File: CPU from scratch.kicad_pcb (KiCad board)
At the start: 2 copper layers, 90 x 35 mm, 50 parts, among them J1 Screw_Terminal_01x03, J2 Screw_Terminal_01x02, Q1 2N3904, Q10 2N3904, Q11 2N3904, Q12 2N3904, Q13 2N3904, Q14 2N3904, Q15 2N3904, Q16 2N3904, Q17 2N3904, Q18 2N3904, Q19 2N3904, Q2 2N3904, Q20 2N3904, Q21 2N3904, Q3 2N3904, Q4 2N3904, Q5 2N3904, Q6 2N3904, Q7 2N3904, Q8 2N3904, Q9 2N3904

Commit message: Update Readme
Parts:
- removed J1: Screw_Terminal_01x03, TerminalBlock_Phoenix:TerminalBlock_Phoenix_MKDS-1,5-3-5.08_1x03_P5.08mm_Horizontal
- removed J2: Screw_Terminal_01x02, TerminalBlock_Phoenix:TerminalBlock_Phoenix_MKDS-1,5-2-5.08_1x02_P5.08mm_Horizontal
- added D1: D, Diode_THT:D_DO-35_SOD27_P7.62mm_Horizontal, F.Cu at (136.9, 49.1)
- added D1: D, Diode_THT:D_DO-35_SOD27_P7.62mm_Horizontal, F.Cu at (136.9, 117.5)
- added D1: D, Diode_THT:D_DO-35_SOD27_P7.62mm_Horizontal, F.Cu at (149.3, 157.2)
- added D2: D, Diode_THT:D_DO-35_SOD27_P7.62mm_Horizontal, F.Cu at (124.9, 45.1)
- added D2: D, Diode_THT:D_DO-35_SOD27_P7.62mm_Horizontal, F.Cu at (161.3, 161.2)
- added D2: D, Diode_THT:D_DO-35_SOD27_P7.62mm_Horizontal, F.Cu at (124.9, 113.5)
- added D3: D, Diode_THT:D_DO-35_SOD27_P7.62mm_Horizontal, F.Cu at (160.6, 141.4)
- added D3: D, Diode_THT:D_DO-35_SOD27_P7.62mm_Horizontal, F.Cu at (125.6, 64.9)
- added D3: D, Diode_THT:D_DO-35_SOD27_P7.62mm_Horizontal, F.Cu at (125.6, 133.3)
- added D4: D, Diode_THT:D_DO-35_SOD27_P7.62mm_Horizontal, F.Cu at (168.8, 48.9)
- added D4: D, Diode_THT:D_DO-35_SOD27_P7.62mm_Horizontal, F.Cu at (168.8, 117.3)
- added D4: D, Diode_THT:D_DO-35_SOD27_P7.62mm_Horizontal, F.Cu at (117.4, 157.4)
- added D5: D, Diode_THT:D_DO-35_SOD27_P7.62mm_Horizontal, F.Cu at (129.4, 161.4)
- added D5: D, Diode_THT:D_DO-35_SOD27_P7.62mm_Horizontal, F.Cu at (156.8, 113.3)
- added D5: D, Diode_THT:D_DO-35_SOD27_P7.62mm_Horizontal, F.Cu at (156.8, 44.9)
- added D6: D, Diode_THT:D_DO-35_SOD27_P7.62mm_Horizontal, F.Cu at (120.6, 141.4)
- added D6: D, Diode_THT:D_DO-35_SOD27_P7.62mm_Horizontal, F.Cu at (165.6, 133.3)
- added D6: D, Diode_THT:D_DO-35_SOD27_P7.62mm_Horizontal, F.Cu at (165.6, 64.9)
- added D7: D, Diode_THT:D_DO-35_SOD27_P7.62mm_Horizontal, F.Cu at (137.6, 141.4)
- added D7: D, Diode_THT:D_DO-35_SOD27_P7.62mm_Horizontal, F.Cu at (148.6, 64.9)
- added D7: D, Diode_THT:D_DO-35_SOD27_P7.62mm_Horizontal, F.Cu at (148.6, 133.3)
- added Q1: 2N3904, Package_TO_SOT_THT:TO-92_Inline, F.Cu at (144.3, 155.7)
- added Q1: 2N3904, Package_TO_SOT_THT:TO-92_Inline, F.Cu at (141.9, 119.0)
- added Q1: 2N3904, Package_TO_SOT_THT:TO-92_Inline, F.Cu at (141.9, 50.6)
- added Q10: 2N3904, Package_TO_SOT_THT:TO-92_Inline, F.Cu at (173.8, 50.3)
- added Q10: 2N3904, Package_TO_SOT_THT:TO-92_Inline, F.Cu at (112.4, 156.0)
- added Q10: 2N3904, Package_TO_SOT_THT:TO-92_Inline, F.Cu at (173.8, 118.7)
- added Q11: 2N3904, Package_TO_SOT_THT:TO-92_Inline, F.Cu at (121.4, 163.0)
- added Q11: 2N3904, Package_TO_SOT_THT:TO-92_Inline, F.Cu at (164.8, 111.7)
- added Q11: 2N3904, Package_TO_SOT_THT:TO-92_Inline, F.Cu at (164.8, 43.3)
- added Q12: 2N3904, Package_TO_SOT_THT:TO-92_Inline, F.Cu at (164.8, 117.7)
- added Q12: 2N3904, Package_TO_SOT_THT:TO-92_Inline, F.Cu at (121.4, 157.0)
- added Q12: 2N3904, Package_TO_SOT_THT:TO-92_Inline, F.Cu at (164.8, 49.3)
- added Q13: 2N3904, Package_TO_SOT_THT:TO-92_Inline, F.Cu at (157.5, 117.5)
- added Q13: 2N3904, Package_TO_SOT_THT:TO-92_Inline, F.Cu at (157.5, 49.1)
- added Q13: 2N3904, Package_TO_SOT_THT:TO-92_Inline, F.Cu at (128.7, 157.2)
- added Q14: 2N3904, Package_TO_SOT_THT:TO-92_Inline, F.Cu at (133.4, 163.0)
- added Q14: 2N3904, Package_TO_SOT_THT:TO-92_Inline, F.Cu at (152.8, 43.3)
- added Q14: 2N3904, Package_TO_SOT_THT:TO-92_Inline, F.Cu at (152.8, 111.7)
- added Q15: 2N3904, Package_TO_SOT_THT:TO-92_Inline, F.Cu at (152.8, 49.3)
- added Q15: 2N3904, Package_TO_SOT_THT:TO-92_Inline, F.Cu at (133.4, 157.0)
- added Q15: 2N3904, Package_TO_SOT_THT:TO-92_Inline, F.Cu at (152.8, 117.7)
- added Q16: 2N3904, Package_TO_SOT_THT:TO-92_Inline, F.Cu at (170.6, 134.8)
- added Q16: 2N3904, Package_TO_SOT_THT:TO-92_Inline, F.Cu at (115.6, 139.9)
- added Q16: 2N3904, Package_TO_SOT_THT:TO-92_Inline, F.Cu at (170.6, 66.4)
- added Q17: 2N3904, Package_TO_SOT_THT:TO-92_Inline, F.Cu at (161.6, 60.1)
- added Q17: 2N3904, Package_TO_SOT_THT:TO-92_Inline, F.Cu at (161.6, 128.5)
- added Q17: 2N3904, Package_TO_SOT_THT:TO-92_Inline, F.Cu at (124.6, 146.2)
- added Q18: 2N3904, Package_TO_SOT_THT:TO-92_Inline, F.Cu at (161.6, 66.4)
- added Q18: 2N3904, Package_TO_SOT_THT:TO-92_Inline, F.Cu at (161.6, 134.8)
- added Q18: 2N3904, Package_TO_SOT_THT:TO-92_Inline, F.Cu at (124.6, 139.9)
- added Q19: 2N3904, Package_TO_SOT_THT:TO-92_Inline, F.Cu at (153.5, 134.8)
- added Q19: 2N3904, Package_TO_SOT_THT:TO-92_Inline, F.Cu at (132.7, 139.9)
- added Q19: 2N3904, Package_TO_SOT_THT:TO-92_Inline, F.Cu at (153.5, 66.4)
- added Q2: 2N3904, Package_TO_SOT_THT:TO-92_Inline, F.Cu at (153.3, 162.7)
- added Q2: 2N3904, Package_TO_SOT_THT:TO-92_Inline, F.Cu at (132.9, 43.6)
- added Q2: 2N3904, Package_TO_SOT_THT:TO-92_Inline, F.Cu at (132.9, 112.0)
- added Q20: 2N3904, Package_TO_SOT_THT:TO-92_Inline, F.Cu at (144.6, 128.3)
- added Q20: 2N3904, Package_TO_SOT_THT:TO-92_Inline, F.Cu at (141.6, 146.4)
- added Q20: 2N3904, Package_TO_SOT_THT:TO-92_Inline, F.Cu at (144.6, 59.9)
- added Q21: 2N3904, Package_TO_SOT_THT:TO-92_Inline, F.Cu at (144.6, 65.9)
- added Q21: 2N3904, Package_TO_SOT_THT:TO-92_Inline, F.Cu at (141.6, 140.4)
- added Q21: 2N3904, Package_TO_SOT_THT:TO-92_Inline, F.Cu at (144.6, 134.3)
- added Q3: 2N3904, Package_TO_SOT_THT:TO-92_Inline, F.Cu at (132.9, 49.6)
- added Q3: 2N3904, Package_TO_SOT_THT:TO-92_Inline, F.Cu at (153.3, 156.7)
- added Q3: 2N3904, Package_TO_SOT_THT:TO-92_Inline, F.Cu at (132.9, 118.0)
- added Q4: 2N3904, Package_TO_SOT_THT:TO-92_Inline, F.Cu at (125.6, 49.3)
- added Q4: 2N3904, Package_TO_SOT_THT:TO-92_Inline, F.Cu at (125.6, 117.7)
- added Q4: 2N3904, Package_TO_SOT_THT:TO-92_Inline, F.Cu at (160.6, 157.0)
- added Q5: 2N3904, Package_TO_SOT_THT:TO-92_Inline, F.Cu at (165.3, 162.5)
- added Q5: 2N3904, Package_TO_SOT_THT:TO-92_Inline, F.Cu at (120.9, 43.8)
- added Q5: 2N3904, Package_TO_SOT_THT:TO-92_Inline, F.Cu at (120.9, 112.2)
- added Q6: 2N3904, Package_TO_SOT_THT:TO-92_Inline, F.Cu at (165.3, 156.5)
- added Q6: 2N3904, Package_TO_SOT_THT:TO-92_Inline, F.Cu at (120.9, 118.2)
- added Q6: 2N3904, Package_TO_SOT_THT:TO-92_Inline, F.Cu at (120.9, 49.8)
- added Q7: 2N3904, Package_TO_SOT_THT:TO-92_Inline, F.Cu at (155.6, 139.9)
- added Q7: 2N3904, Package_TO_SOT_THT:TO-92_Inline, F.Cu at (130.6, 66.4)
- added Q7: 2N3904, Package_TO_SOT_THT:TO-92_Inline, F.Cu at (130.6, 134.8)
- added Q8: 2N3904, Package_TO_SOT_THT:TO-92_Inline, F.Cu at (121.6, 60.1)
- added Q8: 2N3904, Package_TO_SOT_THT:TO-92_Inline, F.Cu at (121.6, 128.5)
- added Q8: 2N3904, Package_TO_SOT_THT:TO-92_Inline, F.Cu at (164.6, 146.2)
- added Q9: 2N3904, Package_TO_SOT_THT:TO-92_Inline, F.Cu at (121.6, 66.1)
- added Q9: 2N3904, Package_TO_SOT_THT:TO-92_Inline, F.Cu at (121.6, 134.5)
- added Q9: 2N3904, Package_TO_SOT_THT:TO-92_Inline, F.Cu at (164.6, 140.2)
- added R1: 1k, Resistor_THT:R_Axial_DIN0207_L6.3mm_D2.5mm_P7.62mm_Horizontal, F.Cu at (115.6, 40.3)
- added R1: 1k, Resistor_THT:R_Axial_DIN0207_L6.3mm_D2.5mm_P7.62mm_Horizontal, F.Cu at (170.6, 166.0)
- added R1: 1k, Resistor_THT:R_Axial_DIN0207_L6.3mm_D2.5mm_P7.62mm_Horizontal, F.Cu at (115.6, 108.7)
- added R10: 1k, Resistor_THT:R_Axial_DIN0207_L6.3mm_D2.5mm_P7.62mm_Horizontal, F.Cu at (114.1, 105.7)
- added R10: 1k, Resistor_THT:R_Axial_DIN0207_L6.3mm_D2.5mm_P7.62mm_Horizontal, F.Cu at (172.1, 169.0)
- added R10: 1k, Resistor_THT:R_Axial_DIN0207_L6.3mm_D2.5mm_P7.62mm_Horizontal, F.Cu at (114.1, 37.3)
- added R11: 1k, Resistor_THT:R_Axial_DIN0207_L6.3mm_D2.5mm_P7.62mm_Horizontal, F.Cu at (126.4, 54.1)
- added R11: 1k, Resistor_THT:R_Axial_DIN0207_L6.3mm_D2.5mm_P7.62mm_Horizontal, F.Cu at (159.7, 152.2)
- added R11: 1k, Resistor_THT:R_Axial_DIN0207_L6.3mm_D2.5mm_P7.62mm_Horizontal, F.Cu at (126.4, 122.5)
- added R12: 1k, Resistor_THT:R_Axial_DIN0207_L6.3mm_D2.5mm_P7.62mm_Horizontal, F.Cu at (130.6, 121.7)
- added R12: 1k, Resistor_THT:R_Axial_DIN0207_L6.3mm_D2.5mm_P7.62mm_Horizontal, F.Cu at (155.6, 153.0)
- added R12: 1k, Resistor_THT:R_Axial_DIN0207_L6.3mm_D2.5mm_P7.62mm_Horizontal, F.Cu at (130.6, 53.3)
- added R13: 1k, Resistor_THT:R_Axial_DIN0207_L6.3mm_D2.5mm_P7.62mm_Horizontal, F.Cu at (170.6, 37.1)
- added R13: 1k, Resistor_THT:R_Axial_DIN0207_L6.3mm_D2.5mm_P7.62mm_Horizontal, F.Cu at (115.6, 169.2)
- added R13: 1k, Resistor_THT:R_Axial_DIN0207_L6.3mm_D2.5mm_P7.62mm_Horizontal, F.Cu at (170.6, 105.5)
- added R14: 1k, Resistor_THT:R_Axial_DIN0207_L6.3mm_D2.5mm_P7.62mm_Horizontal, F.Cu at (173.8, 105.7)
- added R14: 1k, Resistor_THT:R_Axial_DIN0207_L6.3mm_D2.5mm_P7.62mm_Horizontal, F.Cu at (112.4, 169.1)
- added R14: 1k, Resistor_THT:R_Axial_DIN0207_L6.3mm_D2.5mm_P7.62mm_Horizontal, F.Cu at (173.8, 37.3)
- added R15: 1k, Resistor_THT:R_Axial_DIN0207_L6.3mm_D2.5mm_P7.62mm_Horizontal, F.Cu at (159.8, 105.7)
- added R15: 1k, Resistor_THT:R_Axial_DIN0207_L6.3mm_D2.5mm_P7.62mm_Horizontal, F.Cu at (126.4, 169.1)
- added R15: 1k, Resistor_THT:R_Axial_DIN0207_L6.3mm_D2.5mm_P7.62mm_Horizontal, F.Cu at (159.8, 37.3)
- added R16: 1k, Resistor_THT:R_Axial_DIN0207_L6.3mm_D2.5mm_P7.62mm_Horizontal, F.Cu at (140.2, 169.2)
- added R16: 1k, Resistor_THT:R_Axial_DIN0207_L6.3mm_D2.5mm_P7.62mm_Horizontal, F.Cu at (145.9, 105.5)
- added R16: 1k, Resistor_THT:R_Axial_DIN0207_L6.3mm_D2.5mm_P7.62mm_Horizontal, F.Cu at (145.9, 37.1)
- added R17: 1k, Resistor_THT:R_Axial_DIN0207_L6.3mm_D2.5mm_P7.62mm_Horizontal, F.Cu at (166.4, 54.2)
- added R17: 1k, Resistor_THT:R_Axial_DIN0207_L6.3mm_D2.5mm_P7.62mm_Horizontal, F.Cu at (166.4, 122.6)
- added R17: 1k, Resistor_THT:R_Axial_DIN0207_L6.3mm_D2.5mm_P7.62mm_Horizontal, F.Cu at (119.7, 152.1)
- added R18: 1k, Resistor_THT:R_Axial_DIN0207_L6.3mm_D2.5mm_P7.62mm_Horizontal, F.Cu at (170.6, 53.3)
- added R18: 1k, Resistor_THT:R_Axial_DIN0207_L6.3mm_D2.5mm_P7.62mm_Horizontal, F.Cu at (170.6, 121.7)
- added R18: 1k, Resistor_THT:R_Axial_DIN0207_L6.3mm_D2.5mm_P7.62mm_Horizontal, F.Cu at (115.6, 153.0)
- added R19: 1k, Resistor_THT:R_Axial_DIN0207_L6.3mm_D2.5mm_P7.62mm_Horizontal, F.Cu at (148.9, 54.1)
- added R19: 1k, Resistor_THT:R_Axial_DIN0207_L6.3mm_D2.5mm_P7.62mm_Horizontal, F.Cu at (137.2, 152.2)
- added R19: 1k, Resistor_THT:R_Axial_DIN0207_L6.3mm_D2.5mm_P7.62mm_Horizontal, F.Cu at (148.9, 122.5)
- added R2: 1k, Resistor_THT:R_Axial_DIN0207_L6.3mm_D2.5mm_P7.62mm_Horizontal, F.Cu at (111.6, 47.9)
- added R2: 1k, Resistor_THT:R_Axial_DIN0207_L6.3mm_D2.5mm_P7.62mm_Horizontal, F.Cu at (174.6, 158.4)
- added R2: 1k, Resistor_THT:R_Axial_DIN0207_L6.3mm_D2.5mm_P7.62mm_Horizontal, F.Cu at (111.6, 116.3)
- added R20: 1k, Resistor_THT:R_Axial_DIN0207_L6.3mm_D2.5mm_P7.62mm_Horizontal, F.Cu at (153.6, 121.7)
- added R20: 1k, Resistor_THT:R_Axial_DIN0207_L6.3mm_D2.5mm_P7.62mm_Horizontal, F.Cu at (132.6, 153.0)
- added R20: 1k, Resistor_THT:R_Axial_DIN0207_L6.3mm_D2.5mm_P7.62mm_Horizontal, F.Cu at (153.6, 53.3)
- added R3: 1k, Resistor_THT:R_Axial_DIN0207_L6.3mm_D2.5mm_P7.62mm_Horizontal, F.Cu at (147.1, 118.3)
- added R3: 1k, Resistor_THT:R_Axial_DIN0207_L6.3mm_D2.5mm_P7.62mm_Horizontal, F.Cu at (147.1, 49.9)
- added R3: 1k, Resistor_THT:R_Axial_DIN0207_L6.3mm_D2.5mm_P7.62mm_Horizontal, F.Cu at (139.1, 156.4)
- added R4: 1k, Resistor_THT:R_Axial_DIN0207_L6.3mm_D2.5mm_P7.62mm_Horizontal, F.Cu at (170.6, 154.0)
- added R4: 1k, Resistor_THT:R_Axial_DIN0207_L6.3mm_D2.5mm_P7.62mm_Horizontal, F.Cu at (115.6, 52.3)
- added R4: 1k, Resistor_THT:R_Axial_DIN0207_L6.3mm_D2.5mm_P7.62mm_Horizontal, F.Cu at (115.6, 120.7)
- added R5: 1k, Resistor_THT:R_Axial_DIN0207_L6.3mm_D2.5mm_P7.62mm_Horizontal, F.Cu at (174.6, 154.0)
- added R5: 1k, Resistor_THT:R_Axial_DIN0207_L6.3mm_D2.5mm_P7.62mm_Horizontal, F.Cu at (111.6, 120.7)
- added R5: 1k, Resistor_THT:R_Axial_DIN0207_L6.3mm_D2.5mm_P7.62mm_Horizontal, F.Cu at (111.6, 52.3)
- added R6: 1k, Resistor_THT:R_Axial_DIN0207_L6.3mm_D2.5mm_P7.62mm_Horizontal, F.Cu at (148.6, 148.5)
- added R6: 1k, Resistor_THT:R_Axial_DIN0207_L6.3mm_D2.5mm_P7.62mm_Horizontal, F.Cu at (137.6, 126.2)
- added R6: 1k, Resistor_THT:R_Axial_DIN0207_L6.3mm_D2.5mm_P7.62mm_Horizontal, F.Cu at (137.6, 57.8)
- added R7: 1k, Resistor_THT:R_Axial_DIN0207_L6.3mm_D2.5mm_P7.62mm_Horizontal, F.Cu at (138.7, 105.7)
- added R7: 1k, Resistor_THT:R_Axial_DIN0207_L6.3mm_D2.5mm_P7.62mm_Horizontal, F.Cu at (138.7, 37.3)
- added R7: 1k, Resistor_THT:R_Axial_DIN0207_L6.3mm_D2.5mm_P7.62mm_Horizontal, F.Cu at (147.5, 169.0)
- added R8: 1k, Resistor_THT:R_Axial_DIN0207_L6.3mm_D2.5mm_P7.62mm_Horizontal, F.Cu at (141.9, 37.5)
- added R8: 1k, Resistor_THT:R_Axial_DIN0207_L6.3mm_D2.5mm_P7.62mm_Horizontal, F.Cu at (141.9, 105.9)
- added R8: 1k, Resistor_THT:R_Axial_DIN0207_L6.3mm_D2.5mm_P7.62mm_Horizontal, F.Cu at (144.3, 168.8)
- added R9: 1k, Resistor_THT:R_Axial_DIN0207_L6.3mm_D2.5mm_P7.62mm_Horizontal, F.Cu at (158.3, 168.8)
- added R9: 1k, Resistor_THT:R_Axial_DIN0207_L6.3mm_D2.5mm_P7.62mm_Horizontal, F.Cu at (127.9, 105.9)
- added R9: 1k, Resistor_THT:R_Axial_DIN0207_L6.3mm_D2.5mm_P7.62mm_Horizontal, F.Cu at (127.9, 37.5)
- moved R5 70.2 mm to (174.6, 84.4), turned to 90 degrees
- moved R2 69.1 mm to (174.6, 88.7), turned to -90 degrees
- moved R10 66.0 mm to (172.1, 99.4), turned to 180 degrees
- moved Q16 64.6 mm to (115.6, 70.3), turned to -90 degrees
- moved Q9 64.1 mm to (164.6, 70.5), turned to -90 degrees
- moved R4 62.4 mm to (170.6, 84.4), turned to 90 degrees
- moved R1 61.7 mm to (170.6, 96.4), turned to 90 degrees
- moved R14 57.7 mm to (112.4, 99.4), turned to 90 degrees
- moved Q8 57.1 mm to (164.6, 76.5), turned to -90 degrees
- moved D3 56.5 mm to (160.6, 71.7), turned to -90 degrees
- moved Q10 56.3 mm to (112.4, 86.3), turned to -90 degrees
- moved D6 55.3 mm to (120.6, 71.7), turned to -90 degrees
- moved Q18 52.3 mm to (124.6, 70.3), turned to -90 degrees
- moved Q7 52.1 mm to (155.6, 70.3), turned to -90 degrees
- moved R13 51.8 mm to (115.6, 99.6), turned to 0 degrees
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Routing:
- net /AND2/In1: track 42.7 -> 170.9 mm, vias 1 -> 4
- net /AND1/O: track 35.7 -> 142.7 mm
- net Cin: track 50.1 -> 133.4 mm
- net /XOR1/In2: track 24.8 -> 99.4 mm
- net GND: track 0.00 -> 68.1 mm
- net Net-(Q11-E): track 22.4 -> 89.8 mm
- net /XOR2/In2: track 20.7 -> 82.9 mm
- net /XOR1/In1: track 20.6 -> 82.6 mm
- net Net-(D6-A): track 15.9 -> 63.5 mm
- net Net-(D1-A): track 15.8 -> 63.4 mm
- net Net-(D4-A): track 15.7 -> 62.7 mm
- net Net-(Q2-E): track 14.8 -> 59.1 mm
- net /AND1/In2: track 12.0 -> 48.2 mm
- net /AND2/O: track 11.6 -> 46.6 mm
- net Net-(D3-A): track 8.74 -> 34.9 mm
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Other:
- board size 90 x 35 mm -> 76.2 x 144.8 mm
- board text added: "${REFERENCE}"

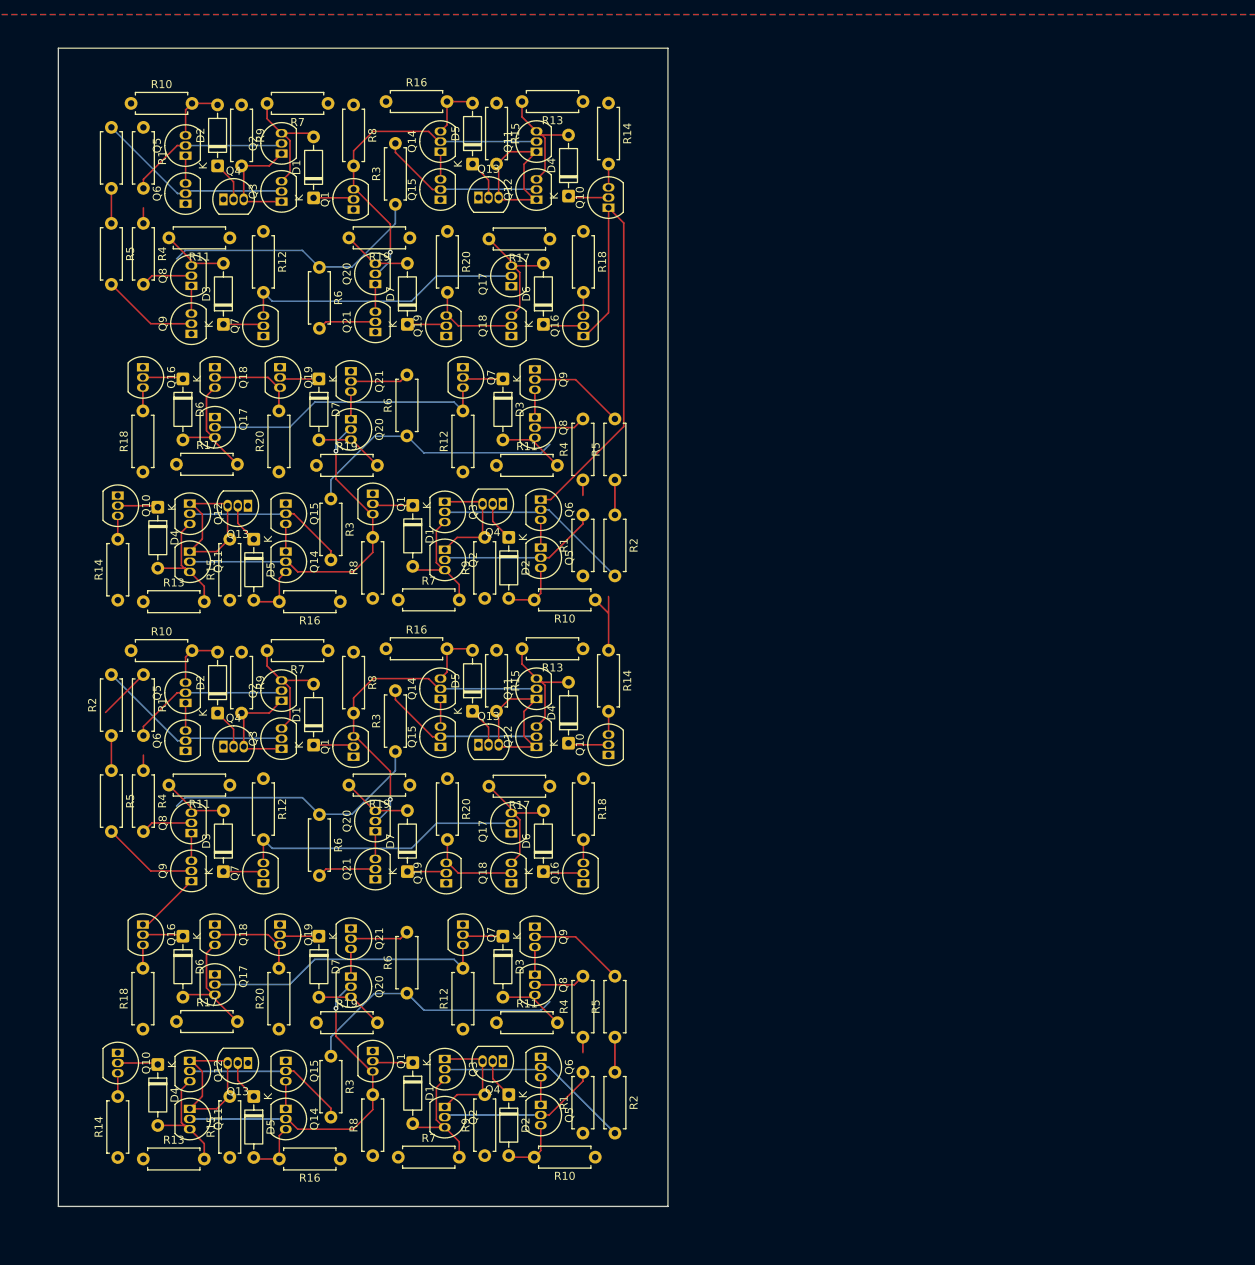
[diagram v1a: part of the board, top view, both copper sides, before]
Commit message: Update Readme
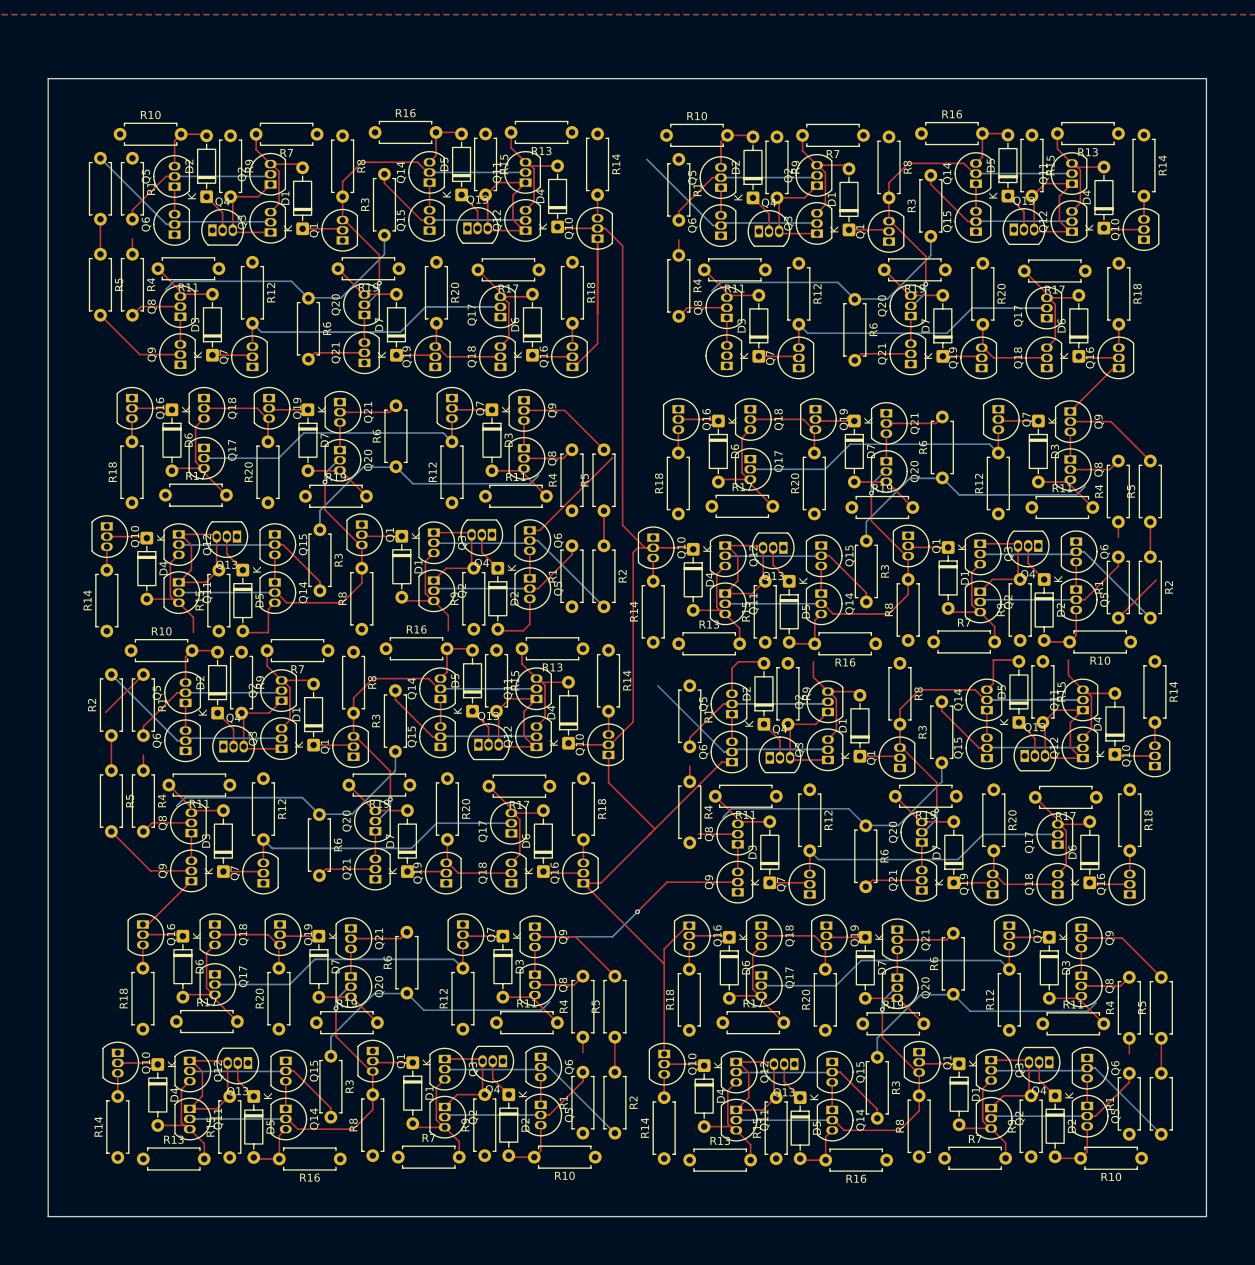
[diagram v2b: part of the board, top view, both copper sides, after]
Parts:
- removed the R10 at (172.1, 99.4)
- removed the R13 at (115.6, 99.6)
- removed the R16 at (140.2, 99.6)
- removed the R7 at (147.5, 99.4)
- added D1: D, Diode_THT:D_DO-35_SOD27_P7.62mm_Horizontal, F.Cu at (217.6, 157.3)
- added D1: D, Diode_THT:D_DO-35_SOD27_P7.62mm_Horizontal, F.Cu at (203.8, 53.1)
- added D1: D, Diode_THT:D_DO-35_SOD27_P7.62mm_Horizontal, F.Cu at (216.2, 92.8)
- added D1: D, Diode_THT:D_DO-35_SOD27_P7.62mm_Horizontal, F.Cu at (205.2, 118.9)
- added D2: D, Diode_THT:D_DO-35_SOD27_P7.62mm_Horizontal, F.Cu at (228.2, 96.8)
- added D2: D, Diode_THT:D_DO-35_SOD27_P7.62mm_Horizontal, F.Cu at (191.8, 49.1)
- added D2: D, Diode_THT:D_DO-35_SOD27_P7.62mm_Horizontal, F.Cu at (193.2, 114.9)
- added D2: D, Diode_THT:D_DO-35_SOD27_P7.62mm_Horizontal, F.Cu at (229.6, 161.3)
- added D3: D, Diode_THT:D_DO-35_SOD27_P7.62mm_Horizontal, F.Cu at (192.5, 68.9)
- added D3: D, Diode_THT:D_DO-35_SOD27_P7.62mm_Horizontal, F.Cu at (193.9, 134.7)
- added D3: D, Diode_THT:D_DO-35_SOD27_P7.62mm_Horizontal, F.Cu at (228.9, 141.5)
- added D3: D, Diode_THT:D_DO-35_SOD27_P7.62mm_Horizontal, F.Cu at (227.5, 77.0)
- added D4: D, Diode_THT:D_DO-35_SOD27_P7.62mm_Horizontal, F.Cu at (237.1, 118.7)
- added D4: D, Diode_THT:D_DO-35_SOD27_P7.62mm_Horizontal, F.Cu at (185.7, 157.6)
- added D4: D, Diode_THT:D_DO-35_SOD27_P7.62mm_Horizontal, F.Cu at (235.7, 52.9)
- added D4: D, Diode_THT:D_DO-35_SOD27_P7.62mm_Horizontal, F.Cu at (184.3, 93.0)
- added D5: D, Diode_THT:D_DO-35_SOD27_P7.62mm_Horizontal, F.Cu at (223.7, 48.9)
- added D5: D, Diode_THT:D_DO-35_SOD27_P7.62mm_Horizontal, F.Cu at (196.3, 97.0)
- added D5: D, Diode_THT:D_DO-35_SOD27_P7.62mm_Horizontal, F.Cu at (225.1, 114.7)
- added D5: D, Diode_THT:D_DO-35_SOD27_P7.62mm_Horizontal, F.Cu at (197.7, 161.6)
- added D6: D, Diode_THT:D_DO-35_SOD27_P7.62mm_Horizontal, F.Cu at (188.9, 141.5)
- added D6: D, Diode_THT:D_DO-35_SOD27_P7.62mm_Horizontal, F.Cu at (233.9, 134.7)
- added D6: D, Diode_THT:D_DO-35_SOD27_P7.62mm_Horizontal, F.Cu at (187.5, 77.0)
- added D6: D, Diode_THT:D_DO-35_SOD27_P7.62mm_Horizontal, F.Cu at (232.5, 68.9)
- added D7: D, Diode_THT:D_DO-35_SOD27_P7.62mm_Horizontal, F.Cu at (204.5, 77.0)
- added D7: D, Diode_THT:D_DO-35_SOD27_P7.62mm_Horizontal, F.Cu at (216.9, 134.7)
- added D7: D, Diode_THT:D_DO-35_SOD27_P7.62mm_Horizontal, F.Cu at (215.5, 68.9)
- added D7: D, Diode_THT:D_DO-35_SOD27_P7.62mm_Horizontal, F.Cu at (205.9, 141.5)
- added Q1: 2N3904, Package_TO_SOT_THT:TO-92_Inline, F.Cu at (208.8, 54.6)
- added Q1: 2N3904, Package_TO_SOT_THT:TO-92_Inline, F.Cu at (211.2, 91.3)
- added Q1: 2N3904, Package_TO_SOT_THT:TO-92_Inline, F.Cu at (210.2, 120.4)
- added Q1: 2N3904, Package_TO_SOT_THT:TO-92_Inline, F.Cu at (212.6, 155.9)
- added Q10: 2N3904, Package_TO_SOT_THT:TO-92_Inline, F.Cu at (242.1, 120.1)
- added Q10: 2N3904, Package_TO_SOT_THT:TO-92_Inline, F.Cu at (179.3, 91.6)
- added Q10: 2N3904, Package_TO_SOT_THT:TO-92_Inline, F.Cu at (180.7, 156.1)
- added Q10: 2N3904, Package_TO_SOT_THT:TO-92_Inline, F.Cu at (240.7, 54.3)
- added Q11: 2N3904, Package_TO_SOT_THT:TO-92_Inline, F.Cu at (189.7, 163.1)
- added Q11: 2N3904, Package_TO_SOT_THT:TO-92_Inline, F.Cu at (188.3, 98.6)
- added Q11: 2N3904, Package_TO_SOT_THT:TO-92_Inline, F.Cu at (231.7, 47.3)
- added Q11: 2N3904, Package_TO_SOT_THT:TO-92_Inline, F.Cu at (233.1, 113.1)
- added Q12: 2N3904, Package_TO_SOT_THT:TO-92_Inline, F.Cu at (188.3, 92.6)
- added Q12: 2N3904, Package_TO_SOT_THT:TO-92_Inline, F.Cu at (231.7, 53.3)
- added Q12: 2N3904, Package_TO_SOT_THT:TO-92_Inline, F.Cu at (233.1, 119.1)
- added Q12: 2N3904, Package_TO_SOT_THT:TO-92_Inline, F.Cu at (189.7, 157.1)
- added Q13: 2N3904, Package_TO_SOT_THT:TO-92_Inline, F.Cu at (225.8, 118.9)
- added Q13: 2N3904, Package_TO_SOT_THT:TO-92_Inline, F.Cu at (224.4, 53.1)
- added Q13: 2N3904, Package_TO_SOT_THT:TO-92_Inline, F.Cu at (197.0, 157.4)
- added Q13: 2N3904, Package_TO_SOT_THT:TO-92_Inline, F.Cu at (195.6, 92.8)
- added Q14: 2N3904, Package_TO_SOT_THT:TO-92_Inline, F.Cu at (221.1, 113.1)
- added Q14: 2N3904, Package_TO_SOT_THT:TO-92_Inline, F.Cu at (200.3, 98.6)
- added Q14: 2N3904, Package_TO_SOT_THT:TO-92_Inline, F.Cu at (201.7, 163.1)
- added Q14: 2N3904, Package_TO_SOT_THT:TO-92_Inline, F.Cu at (219.7, 47.3)
- added Q15: 2N3904, Package_TO_SOT_THT:TO-92_Inline, F.Cu at (219.7, 53.3)
- added Q15: 2N3904, Package_TO_SOT_THT:TO-92_Inline, F.Cu at (221.1, 119.1)
- added Q15: 2N3904, Package_TO_SOT_THT:TO-92_Inline, F.Cu at (201.7, 157.1)
- added Q15: 2N3904, Package_TO_SOT_THT:TO-92_Inline, F.Cu at (200.3, 92.6)
- added Q16: 2N3904, Package_TO_SOT_THT:TO-92_Inline, F.Cu at (183.9, 140.1)
- added Q16: 2N3904, Package_TO_SOT_THT:TO-92_Inline, F.Cu at (237.5, 70.4)
- added Q16: 2N3904, Package_TO_SOT_THT:TO-92_Inline, F.Cu at (238.9, 136.2)
- added Q16: 2N3904, Package_TO_SOT_THT:TO-92_Inline, F.Cu at (182.5, 75.5)
- added Q17: 2N3904, Package_TO_SOT_THT:TO-92_Inline, F.Cu at (229.9, 129.9)
- added Q17: 2N3904, Package_TO_SOT_THT:TO-92_Inline, F.Cu at (191.5, 81.8)
- added Q17: 2N3904, Package_TO_SOT_THT:TO-92_Inline, F.Cu at (192.9, 146.3)
- added Q17: 2N3904, Package_TO_SOT_THT:TO-92_Inline, F.Cu at (228.5, 64.1)
- added Q18: 2N3904, Package_TO_SOT_THT:TO-92_Inline, F.Cu at (229.9, 136.2)
- added Q18: 2N3904, Package_TO_SOT_THT:TO-92_Inline, F.Cu at (191.5, 75.5)
- added Q18: 2N3904, Package_TO_SOT_THT:TO-92_Inline, F.Cu at (192.9, 140.1)
- added Q18: 2N3904, Package_TO_SOT_THT:TO-92_Inline, F.Cu at (228.5, 70.4)
- added Q19: 2N3904, Package_TO_SOT_THT:TO-92_Inline, F.Cu at (220.4, 70.4)
- added Q19: 2N3904, Package_TO_SOT_THT:TO-92_Inline, F.Cu at (221.8, 136.2)
- added Q19: 2N3904, Package_TO_SOT_THT:TO-92_Inline, F.Cu at (201.0, 140.1)
- added Q19: 2N3904, Package_TO_SOT_THT:TO-92_Inline, F.Cu at (199.6, 75.5)
- added Q2: 2N3904, Package_TO_SOT_THT:TO-92_Inline, F.Cu at (220.2, 98.3)
- added Q2: 2N3904, Package_TO_SOT_THT:TO-92_Inline, F.Cu at (199.8, 47.6)
- added Q2: 2N3904, Package_TO_SOT_THT:TO-92_Inline, F.Cu at (201.2, 113.4)
- added Q2: 2N3904, Package_TO_SOT_THT:TO-92_Inline, F.Cu at (221.6, 162.9)
- added Q20: 2N3904, Package_TO_SOT_THT:TO-92_Inline, F.Cu at (211.5, 63.9)
- added Q20: 2N3904, Package_TO_SOT_THT:TO-92_Inline, F.Cu at (208.5, 82.0)
- added Q20: 2N3904, Package_TO_SOT_THT:TO-92_Inline, F.Cu at (212.9, 129.7)
- added Q20: 2N3904, Package_TO_SOT_THT:TO-92_Inline, F.Cu at (209.9, 146.6)
- added Q21: 2N3904, Package_TO_SOT_THT:TO-92_Inline, F.Cu at (209.9, 140.6)
- added Q21: 2N3904, Package_TO_SOT_THT:TO-92_Inline, F.Cu at (212.9, 135.7)
- added Q21: 2N3904, Package_TO_SOT_THT:TO-92_Inline, F.Cu at (211.5, 69.9)
- added Q21: 2N3904, Package_TO_SOT_THT:TO-92_Inline, F.Cu at (208.5, 76.0)
- added Q3: 2N3904, Package_TO_SOT_THT:TO-92_Inline, F.Cu at (201.2, 119.4)
- added Q3: 2N3904, Package_TO_SOT_THT:TO-92_Inline, F.Cu at (221.6, 156.9)
- added Q3: 2N3904, Package_TO_SOT_THT:TO-92_Inline, F.Cu at (199.8, 53.6)
- added Q3: 2N3904, Package_TO_SOT_THT:TO-92_Inline, F.Cu at (220.2, 92.3)
- added Q4: 2N3904, Package_TO_SOT_THT:TO-92_Inline, F.Cu at (228.9, 157.2)
- added Q4: 2N3904, Package_TO_SOT_THT:TO-92_Inline, F.Cu at (193.9, 119.1)
- added Q4: 2N3904, Package_TO_SOT_THT:TO-92_Inline, F.Cu at (227.5, 92.6)
- added Q4: 2N3904, Package_TO_SOT_THT:TO-92_Inline, F.Cu at (192.5, 53.3)
- added Q5: 2N3904, Package_TO_SOT_THT:TO-92_Inline, F.Cu at (187.8, 47.8)
- added Q5: 2N3904, Package_TO_SOT_THT:TO-92_Inline, F.Cu at (189.2, 113.6)
- added Q5: 2N3904, Package_TO_SOT_THT:TO-92_Inline, F.Cu at (233.6, 162.6)
- added Q5: 2N3904, Package_TO_SOT_THT:TO-92_Inline, F.Cu at (232.2, 98.1)
- added Q6: 2N3904, Package_TO_SOT_THT:TO-92_Inline, F.Cu at (233.6, 156.6)
- added Q6: 2N3904, Package_TO_SOT_THT:TO-92_Inline, F.Cu at (187.8, 53.8)
- added Q6: 2N3904, Package_TO_SOT_THT:TO-92_Inline, F.Cu at (232.2, 92.1)
- added Q6: 2N3904, Package_TO_SOT_THT:TO-92_Inline, F.Cu at (189.2, 119.6)
- added Q7: 2N3904, Package_TO_SOT_THT:TO-92_Inline, F.Cu at (198.9, 136.2)
- added Q7: 2N3904, Package_TO_SOT_THT:TO-92_Inline, F.Cu at (222.5, 75.5)
- added Q7: 2N3904, Package_TO_SOT_THT:TO-92_Inline, F.Cu at (197.5, 70.4)
- added Q7: 2N3904, Package_TO_SOT_THT:TO-92_Inline, F.Cu at (223.9, 140.1)
- added Q8: 2N3904, Package_TO_SOT_THT:TO-92_Inline, F.Cu at (232.9, 146.3)
- added Q8: 2N3904, Package_TO_SOT_THT:TO-92_Inline, F.Cu at (189.9, 129.9)
- added Q8: 2N3904, Package_TO_SOT_THT:TO-92_Inline, F.Cu at (188.5, 64.1)
- added Q8: 2N3904, Package_TO_SOT_THT:TO-92_Inline, F.Cu at (231.5, 81.8)
- added Q9: 2N3904, Package_TO_SOT_THT:TO-92_Inline, F.Cu at (232.9, 140.3)
- added Q9: 2N3904, Package_TO_SOT_THT:TO-92_Inline, F.Cu at (189.9, 135.9)
- added Q9: 2N3904, Package_TO_SOT_THT:TO-92_Inline, F.Cu at (231.5, 75.8)
- added Q9: 2N3904, Package_TO_SOT_THT:TO-92_Inline, F.Cu at (188.5, 70.1)
- added R1: 1k, Resistor_THT:R_Axial_DIN0207_L6.3mm_D2.5mm_P7.62mm_Horizontal, F.Cu at (182.5, 44.3)
- added R1: 1k, Resistor_THT:R_Axial_DIN0207_L6.3mm_D2.5mm_P7.62mm_Horizontal, F.Cu at (183.9, 110.1)
- added R1: 1k, Resistor_THT:R_Axial_DIN0207_L6.3mm_D2.5mm_P7.62mm_Horizontal, F.Cu at (237.5, 101.6)
- added R1: 1k, Resistor_THT:R_Axial_DIN0207_L6.3mm_D2.5mm_P7.62mm_Horizontal, F.Cu at (238.9, 166.2)
- added R10: 1k, Resistor_THT:R_Axial_DIN0207_L6.3mm_D2.5mm_P7.62mm_Horizontal, F.Cu at (239.0, 104.6)
- added R10: 1k, Resistor_THT:R_Axial_DIN0207_L6.3mm_D2.5mm_P7.62mm_Horizontal, F.Cu at (181.0, 41.3)
- added R10: 1k, Resistor_THT:R_Axial_DIN0207_L6.3mm_D2.5mm_P7.62mm_Horizontal, F.Cu at (240.4, 169.2)
- added R11: 1k, Resistor_THT:R_Axial_DIN0207_L6.3mm_D2.5mm_P7.62mm_Horizontal, F.Cu at (228.0, 152.3)
- added R11: 1k, Resistor_THT:R_Axial_DIN0207_L6.3mm_D2.5mm_P7.62mm_Horizontal, F.Cu at (193.4, 58.1)
- added R11: 1k, Resistor_THT:R_Axial_DIN0207_L6.3mm_D2.5mm_P7.62mm_Horizontal, F.Cu at (226.7, 87.8)
- added R11: 1k, Resistor_THT:R_Axial_DIN0207_L6.3mm_D2.5mm_P7.62mm_Horizontal, F.Cu at (194.7, 123.9)
- added R12: 1k, Resistor_THT:R_Axial_DIN0207_L6.3mm_D2.5mm_P7.62mm_Horizontal, F.Cu at (197.5, 57.3)
- added R12: 1k, Resistor_THT:R_Axial_DIN0207_L6.3mm_D2.5mm_P7.62mm_Horizontal, F.Cu at (222.5, 88.6)
- added R12: 1k, Resistor_THT:R_Axial_DIN0207_L6.3mm_D2.5mm_P7.62mm_Horizontal, F.Cu at (223.9, 153.2)
- added R12: 1k, Resistor_THT:R_Axial_DIN0207_L6.3mm_D2.5mm_P7.62mm_Horizontal, F.Cu at (198.9, 123.1)
- added R13: 1k, Resistor_THT:R_Axial_DIN0207_L6.3mm_D2.5mm_P7.62mm_Horizontal, F.Cu at (183.9, 169.4)
- added R13: 1k, Resistor_THT:R_Axial_DIN0207_L6.3mm_D2.5mm_P7.62mm_Horizontal, F.Cu at (237.5, 41.1)
- added R13: 1k, Resistor_THT:R_Axial_DIN0207_L6.3mm_D2.5mm_P7.62mm_Horizontal, F.Cu at (182.5, 104.8)
- added R14: 1k, Resistor_THT:R_Axial_DIN0207_L6.3mm_D2.5mm_P7.62mm_Horizontal, F.Cu at (240.7, 41.3)
- added R14: 1k, Resistor_THT:R_Axial_DIN0207_L6.3mm_D2.5mm_P7.62mm_Horizontal, F.Cu at (242.1, 107.1)
- added R14: 1k, Resistor_THT:R_Axial_DIN0207_L6.3mm_D2.5mm_P7.62mm_Horizontal, F.Cu at (179.3, 104.7)
- added R14: 1k, Resistor_THT:R_Axial_DIN0207_L6.3mm_D2.5mm_P7.62mm_Horizontal, F.Cu at (180.7, 169.2)
- added R15: 1k, Resistor_THT:R_Axial_DIN0207_L6.3mm_D2.5mm_P7.62mm_Horizontal, F.Cu at (226.7, 41.3)
- added R15: 1k, Resistor_THT:R_Axial_DIN0207_L6.3mm_D2.5mm_P7.62mm_Horizontal, F.Cu at (228.1, 107.1)
- added R15: 1k, Resistor_THT:R_Axial_DIN0207_L6.3mm_D2.5mm_P7.62mm_Horizontal, F.Cu at (194.7, 169.2)
- added R15: 1k, Resistor_THT:R_Axial_DIN0207_L6.3mm_D2.5mm_P7.62mm_Horizontal, F.Cu at (193.3, 104.7)
- added R16: 1k, Resistor_THT:R_Axial_DIN0207_L6.3mm_D2.5mm_P7.62mm_Horizontal, F.Cu at (208.5, 169.4)
- added R16: 1k, Resistor_THT:R_Axial_DIN0207_L6.3mm_D2.5mm_P7.62mm_Horizontal, F.Cu at (207.2, 104.8)
- added R16: 1k, Resistor_THT:R_Axial_DIN0207_L6.3mm_D2.5mm_P7.62mm_Horizontal, F.Cu at (212.9, 41.1)
- added R17: 1k, Resistor_THT:R_Axial_DIN0207_L6.3mm_D2.5mm_P7.62mm_Horizontal, F.Cu at (233.4, 58.2)
- added R17: 1k, Resistor_THT:R_Axial_DIN0207_L6.3mm_D2.5mm_P7.62mm_Horizontal, F.Cu at (188.0, 152.2)
- added R17: 1k, Resistor_THT:R_Axial_DIN0207_L6.3mm_D2.5mm_P7.62mm_Horizontal, F.Cu at (234.7, 124.0)
- added R17: 1k, Resistor_THT:R_Axial_DIN0207_L6.3mm_D2.5mm_P7.62mm_Horizontal, F.Cu at (186.7, 87.7)
- added R18: 1k, Resistor_THT:R_Axial_DIN0207_L6.3mm_D2.5mm_P7.62mm_Horizontal, F.Cu at (237.5, 57.3)
- added R18: 1k, Resistor_THT:R_Axial_DIN0207_L6.3mm_D2.5mm_P7.62mm_Horizontal, F.Cu at (182.5, 88.6)
- added R18: 1k, Resistor_THT:R_Axial_DIN0207_L6.3mm_D2.5mm_P7.62mm_Horizontal, F.Cu at (238.9, 123.1)
- added R18: 1k, Resistor_THT:R_Axial_DIN0207_L6.3mm_D2.5mm_P7.62mm_Horizontal, F.Cu at (183.9, 153.2)
- added R19: 1k, Resistor_THT:R_Axial_DIN0207_L6.3mm_D2.5mm_P7.62mm_Horizontal, F.Cu at (204.2, 87.8)
- added R19: 1k, Resistor_THT:R_Axial_DIN0207_L6.3mm_D2.5mm_P7.62mm_Horizontal, F.Cu at (215.9, 58.1)
- added R19: 1k, Resistor_THT:R_Axial_DIN0207_L6.3mm_D2.5mm_P7.62mm_Horizontal, F.Cu at (217.2, 123.9)
- added R19: 1k, Resistor_THT:R_Axial_DIN0207_L6.3mm_D2.5mm_P7.62mm_Horizontal, F.Cu at (205.5, 152.3)
- added R2: 1k, Resistor_THT:R_Axial_DIN0207_L6.3mm_D2.5mm_P7.62mm_Horizontal, F.Cu at (241.5, 94.0)
- added R2: 1k, Resistor_THT:R_Axial_DIN0207_L6.3mm_D2.5mm_P7.62mm_Horizontal, F.Cu at (242.9, 158.5)
- added R20: 1k, Resistor_THT:R_Axial_DIN0207_L6.3mm_D2.5mm_P7.62mm_Horizontal, F.Cu at (199.5, 88.6)
- added R20: 1k, Resistor_THT:R_Axial_DIN0207_L6.3mm_D2.5mm_P7.62mm_Horizontal, F.Cu at (221.9, 123.1)
- added R20: 1k, Resistor_THT:R_Axial_DIN0207_L6.3mm_D2.5mm_P7.62mm_Horizontal, F.Cu at (200.9, 153.2)
- added R20: 1k, Resistor_THT:R_Axial_DIN0207_L6.3mm_D2.5mm_P7.62mm_Horizontal, F.Cu at (220.5, 57.3)
- added R3: 1k, Resistor_THT:R_Axial_DIN0207_L6.3mm_D2.5mm_P7.62mm_Horizontal, F.Cu at (207.4, 156.5)
- added R3: 1k, Resistor_THT:R_Axial_DIN0207_L6.3mm_D2.5mm_P7.62mm_Horizontal, F.Cu at (206.0, 92.0)
- added R3: 1k, Resistor_THT:R_Axial_DIN0207_L6.3mm_D2.5mm_P7.62mm_Horizontal, F.Cu at (215.4, 119.7)
- added R3: 1k, Resistor_THT:R_Axial_DIN0207_L6.3mm_D2.5mm_P7.62mm_Horizontal, F.Cu at (214.0, 53.9)
- added R4: 1k, Resistor_THT:R_Axial_DIN0207_L6.3mm_D2.5mm_P7.62mm_Horizontal, F.Cu at (237.5, 89.6)
- added R4: 1k, Resistor_THT:R_Axial_DIN0207_L6.3mm_D2.5mm_P7.62mm_Horizontal, F.Cu at (183.9, 122.1)
- added R4: 1k, Resistor_THT:R_Axial_DIN0207_L6.3mm_D2.5mm_P7.62mm_Horizontal, F.Cu at (238.9, 154.2)
- added R4: 1k, Resistor_THT:R_Axial_DIN0207_L6.3mm_D2.5mm_P7.62mm_Horizontal, F.Cu at (182.5, 56.3)
- added R5: 1k, Resistor_THT:R_Axial_DIN0207_L6.3mm_D2.5mm_P7.62mm_Horizontal, F.Cu at (242.9, 154.2)
- added R5: 1k, Resistor_THT:R_Axial_DIN0207_L6.3mm_D2.5mm_P7.62mm_Horizontal, F.Cu at (241.5, 89.6)
- added R6: 1k, Resistor_THT:R_Axial_DIN0207_L6.3mm_D2.5mm_P7.62mm_Horizontal, F.Cu at (215.5, 84.1)
- added R6: 1k, Resistor_THT:R_Axial_DIN0207_L6.3mm_D2.5mm_P7.62mm_Horizontal, F.Cu at (205.9, 127.6)
- added R6: 1k, Resistor_THT:R_Axial_DIN0207_L6.3mm_D2.5mm_P7.62mm_Horizontal, F.Cu at (204.5, 61.8)
- added R6: 1k, Resistor_THT:R_Axial_DIN0207_L6.3mm_D2.5mm_P7.62mm_Horizontal, F.Cu at (216.9, 148.7)
- added R7: 1k, Resistor_THT:R_Axial_DIN0207_L6.3mm_D2.5mm_P7.62mm_Horizontal, F.Cu at (215.8, 169.2)
- added R7: 1k, Resistor_THT:R_Axial_DIN0207_L6.3mm_D2.5mm_P7.62mm_Horizontal, F.Cu at (214.4, 104.6)
- added R7: 1k, Resistor_THT:R_Axial_DIN0207_L6.3mm_D2.5mm_P7.62mm_Horizontal, F.Cu at (205.6, 41.3)
- added R8: 1k, Resistor_THT:R_Axial_DIN0207_L6.3mm_D2.5mm_P7.62mm_Horizontal, F.Cu at (211.2, 104.4)
- added R8: 1k, Resistor_THT:R_Axial_DIN0207_L6.3mm_D2.5mm_P7.62mm_Horizontal, F.Cu at (210.2, 107.3)
- added R8: 1k, Resistor_THT:R_Axial_DIN0207_L6.3mm_D2.5mm_P7.62mm_Horizontal, F.Cu at (208.8, 41.5)
- added R8: 1k, Resistor_THT:R_Axial_DIN0207_L6.3mm_D2.5mm_P7.62mm_Horizontal, F.Cu at (212.6, 169.0)
- added R9: 1k, Resistor_THT:R_Axial_DIN0207_L6.3mm_D2.5mm_P7.62mm_Horizontal, F.Cu at (225.2, 104.4)
- added R9: 1k, Resistor_THT:R_Axial_DIN0207_L6.3mm_D2.5mm_P7.62mm_Horizontal, F.Cu at (194.8, 41.5)
- added R9: 1k, Resistor_THT:R_Axial_DIN0207_L6.3mm_D2.5mm_P7.62mm_Horizontal, F.Cu at (226.6, 169.0)
- added R9: 1k, Resistor_THT:R_Axial_DIN0207_L6.3mm_D2.5mm_P7.62mm_Horizontal, F.Cu at (196.2, 107.3)
- moved R14 4.10 mm to (111.0, 103.3)
- moved R15 4.10 mm to (125.0, 103.3)
- moved Q10 4.10 mm to (172.4, 54.2)
- moved Q11 4.10 mm to (163.4, 47.2)
- moved Q12 4.10 mm to (163.4, 53.2)
- moved Q14 4.10 mm to (151.4, 47.2)
- moved Q15 4.10 mm to (151.4, 53.2)
- moved Q5 4.10 mm to (119.5, 47.7)
- moved Q6 4.10 mm to (119.5, 53.7)
- moved Q13 4.10 mm to (127.3, 91.4)
- moved D1 4.10 mm to (135.5, 53.0)
- moved D1 4.10 mm to (147.9, 91.4)
- moved D2 4.10 mm to (123.5, 49.0)
- moved D2 4.10 mm to (159.9, 95.4)
- moved D3 4.10 mm to (124.2, 68.8)
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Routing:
- net /AND2/In1: track 170.9 -> 341.8 mm, vias 4 -> 8
- net /AND1/O: track 142.7 -> 285.4 mm
- net Cin: track 133.4 -> 266.8 mm
- net /XOR1/In2: track 99.4 -> 198.8 mm
- net Net-(D4-K): track 20.3 -> 112.8 mm
- net Net-(Q11-E): track 89.8 -> 179.5 mm
- net /XOR2/In2: track 82.9 -> 165.9 mm
- net /XOR1/In1: track 82.6 -> 165.1 mm
- net Net-(D6-A): track 63.5 -> 127.1 mm
- net Net-(D1-A): track 63.4 -> 126.7 mm
- net Net-(D4-A): track 62.7 -> 125.4 mm
- net Net-(Q2-E): track 59.1 -> 118.3 mm
- net GND: track 68.1 -> 126.3 mm
- net /AND1/In2: track 48.2 -> 100.4 mm, vias 0 -> 1
- net /AND2/O: track 46.6 -> 93.2 mm
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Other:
- board size 76.2 x 144.8 mm -> 144.8 x 142.2 mm
